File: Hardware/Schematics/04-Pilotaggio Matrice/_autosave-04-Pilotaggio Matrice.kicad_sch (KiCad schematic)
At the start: 241 parts, among them J1 Conn_02x32_Odd_Even, J2 Conn_02x32_Odd_Even, J3 Conn_02x32_Odd_Even, U1 CD74HC4067M, U10 AD8604ARUZ, U11 AD8604ARUZ, U12 AD8604ARUZ, U13 AD8604ARUZ, U14 AD8604ARUZ, U15 AD8604ARUZ, U16 AD8604ARUZ, U17 AD8604ARUZ, U18 AD8604ARUZ, U19 AD8604ARUZ, U2 CD74HC4067M, U20 CD74HC4067M, U21 AD8604ARUZ, U22 CD74HC4067M, U23 AD8604ARUZ, U25 AD8604ARUZ, U3 CD74HC4067M, U4 CD74HC4067M, U5 CD74HC4067M, U6 CD74HC4067M, U69A AD8604ARUZ, U7 AD8604ARUZ, U8 AD8604ARUZ, U9 AD8604ARUZ

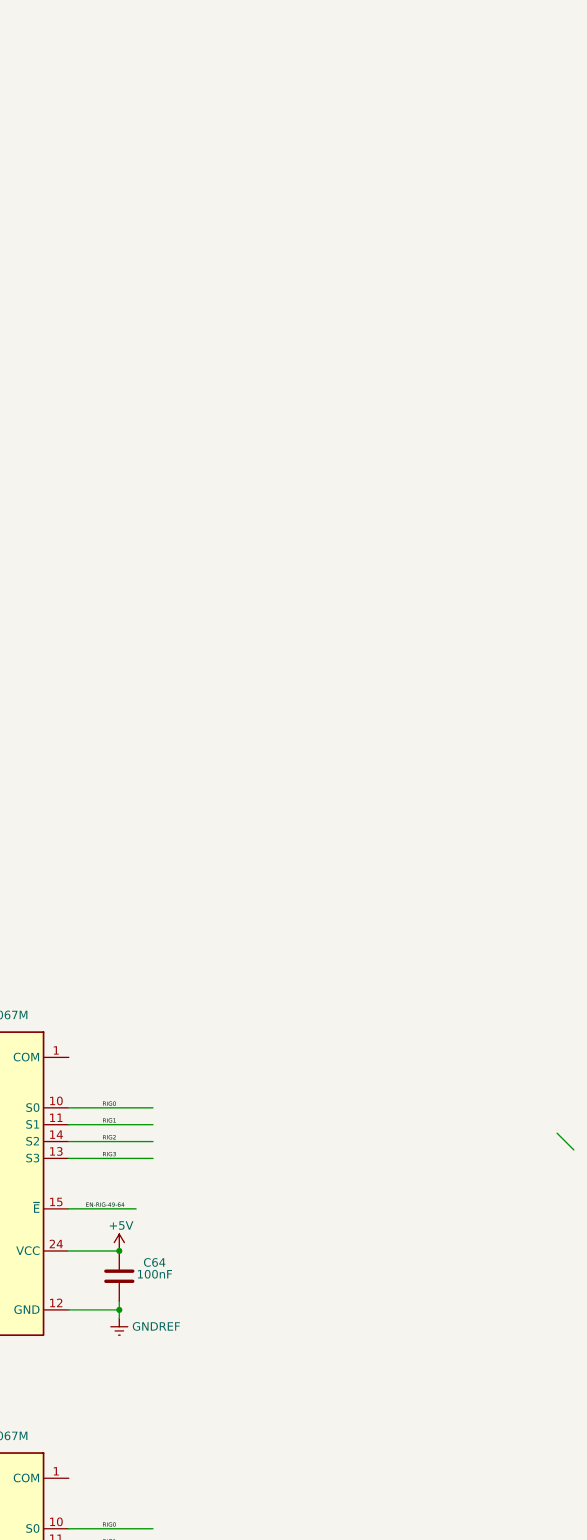
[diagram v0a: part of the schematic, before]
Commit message: update
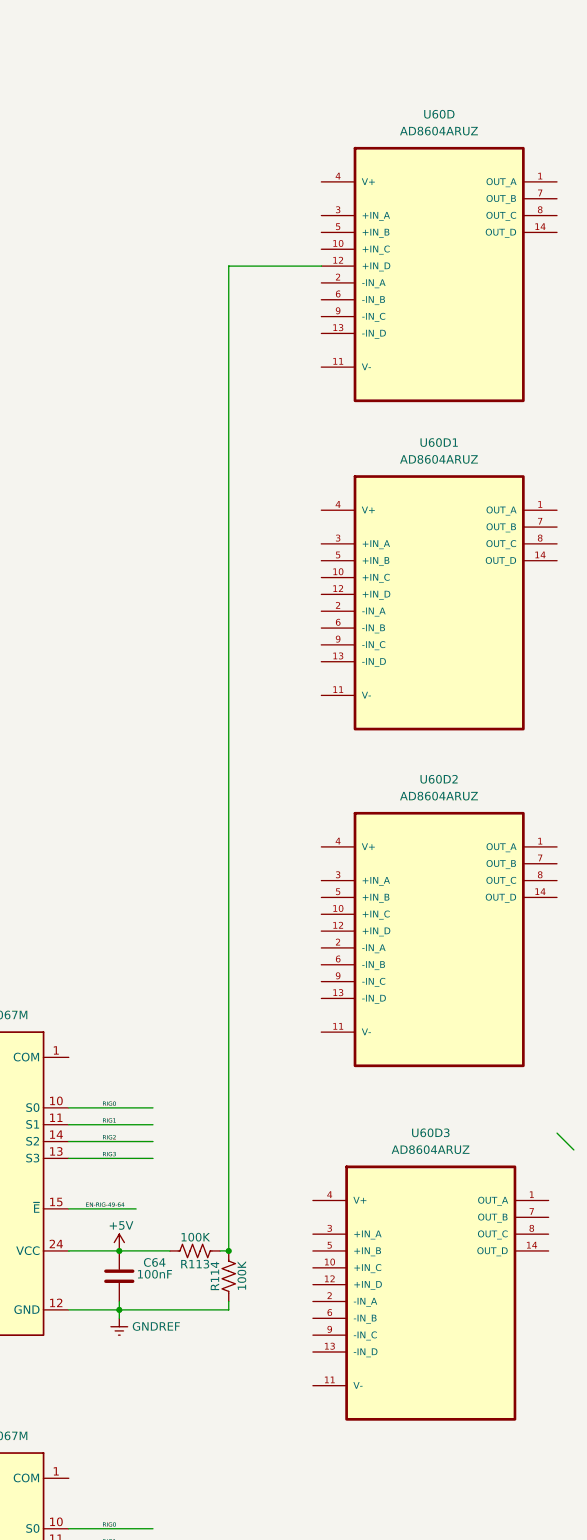
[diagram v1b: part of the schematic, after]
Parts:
- added R113, R114: 100K, symbol Device:R_US
- added U60D, U60D1, U60D2, U60D3: AD8604ARUZ, AD8604ARUZ:SOP65P640X120-14N, symbol AD8604ARUZ:AD8604ARUZ
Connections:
- net +5V: now also R113.1
- net GNDREF: now also R114.2
- new net: R113.2, R114.1, U60D.12 (+IN_D)
